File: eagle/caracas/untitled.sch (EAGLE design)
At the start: 12 parts, among them IC1 4027N, Q1 IRFP250

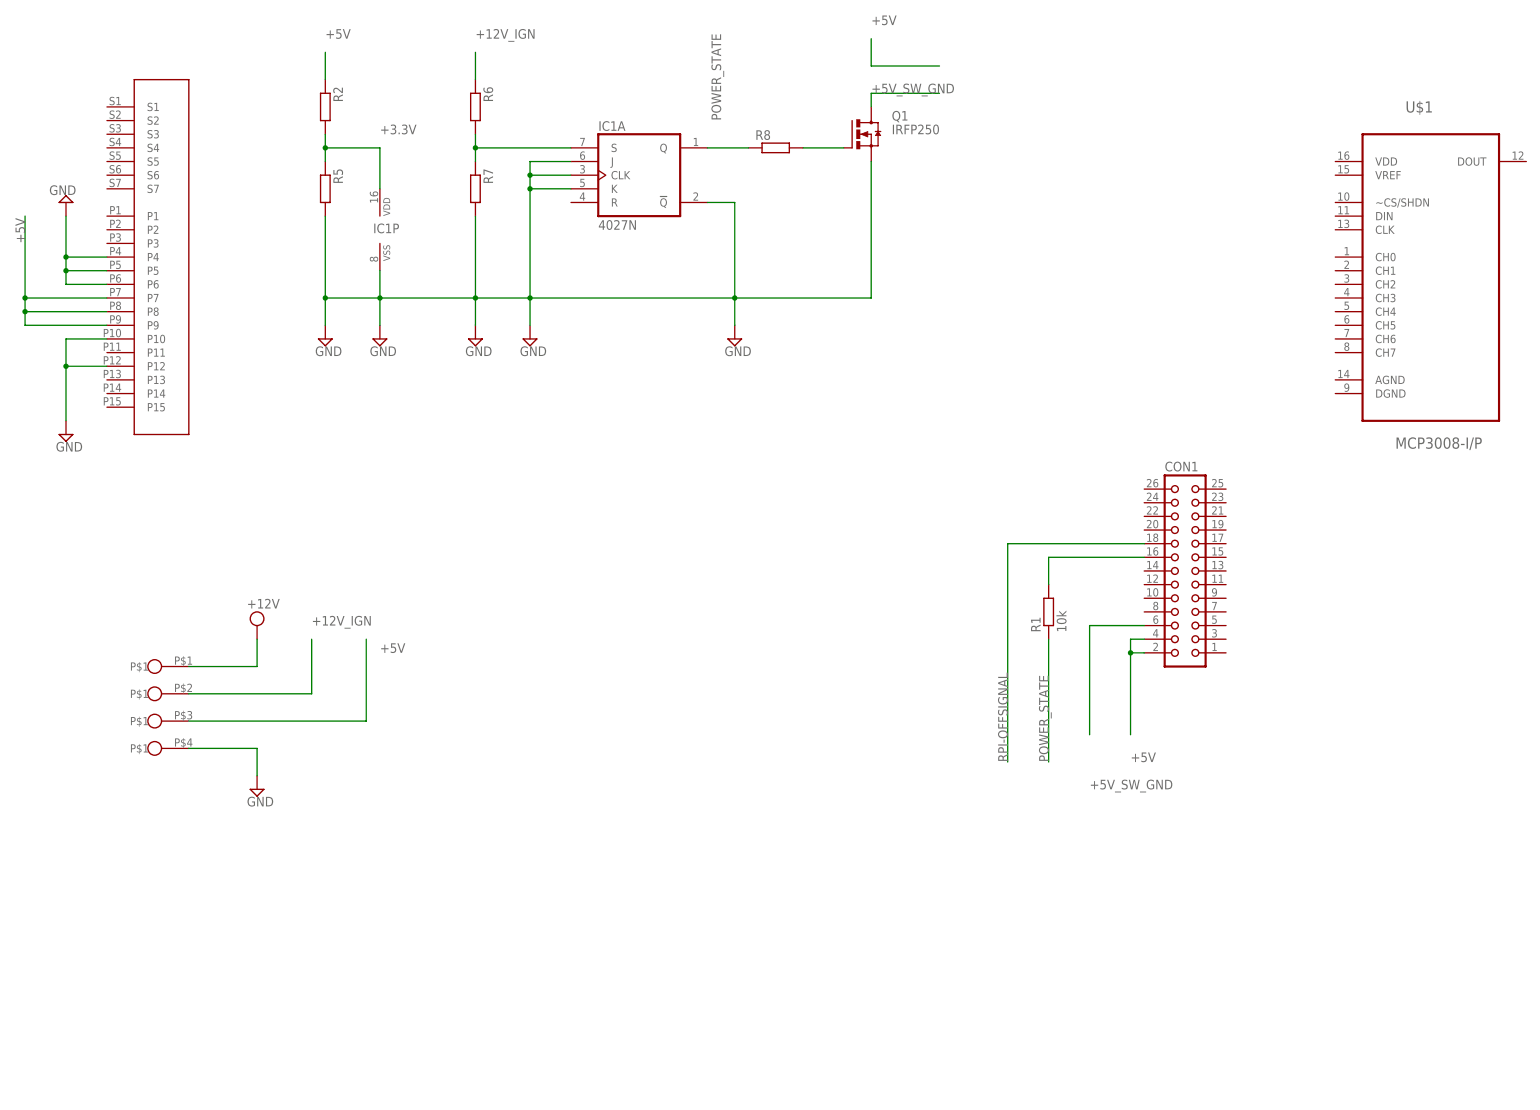
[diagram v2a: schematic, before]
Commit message: WIP on electronics schema.
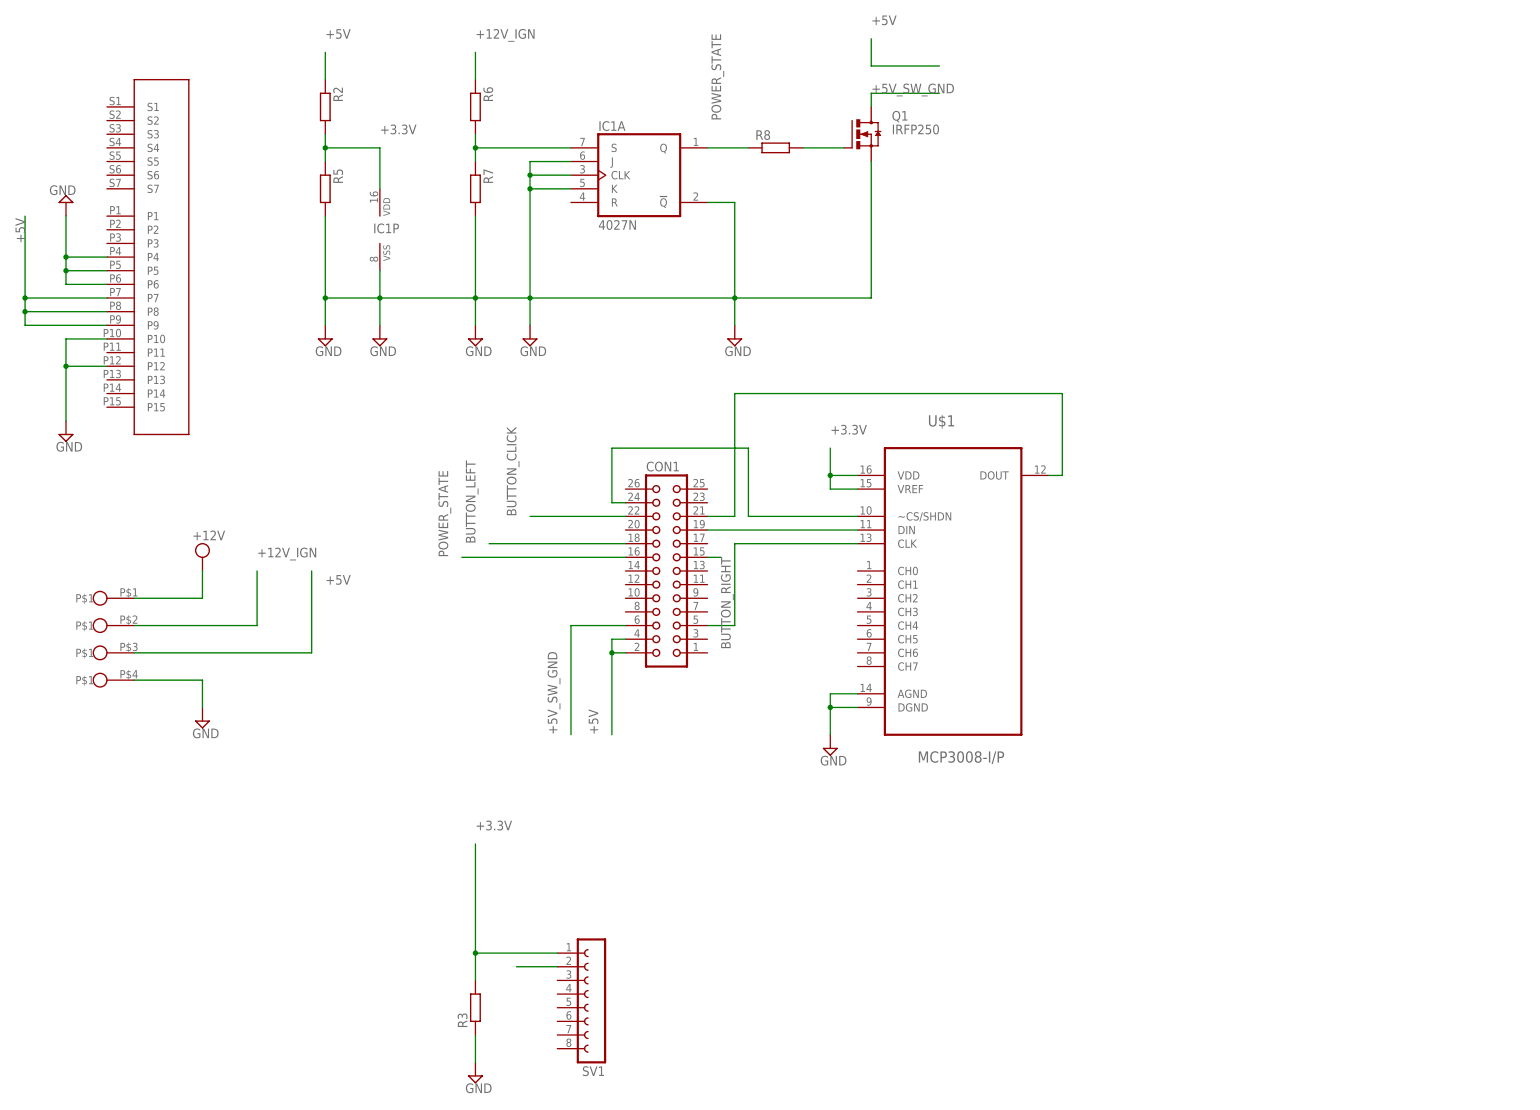
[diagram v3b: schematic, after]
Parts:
- removed R1: 10k, rcl:R-EU_0207/10
- added R3: (no value), rcl:R-EU_0207/10
- added SV1: (no value), con-lsta:FE08-1
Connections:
- net RPI-OFFSIGNAL renamed BUTTON_LEFT
- new net BUTTON_CLICK: CON1.22
- new net BUTTON_RIGHT: CON1.15
- new net N$4: CON1.21, U$1.DOUT
- new net N$5: CON1.19, U$1.DIN
- new net N$6: CON1.24, U$1.~CS/SHDN
- new net N$7: R3.2, SV1.1
- new net N$8: SV1.2
- net +3.3V: now also U$1.VDD, U$1.VREF
- net GND: now also R3.1, U$1.AGND, U$1.DGND
- net N$3: now also CON1.5, U$1.CLK; no longer CON1.16, R1.2
- net POWER_STATE: now also CON1.16; no longer R1.1
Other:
- moved on the sheet: CON1, U$1

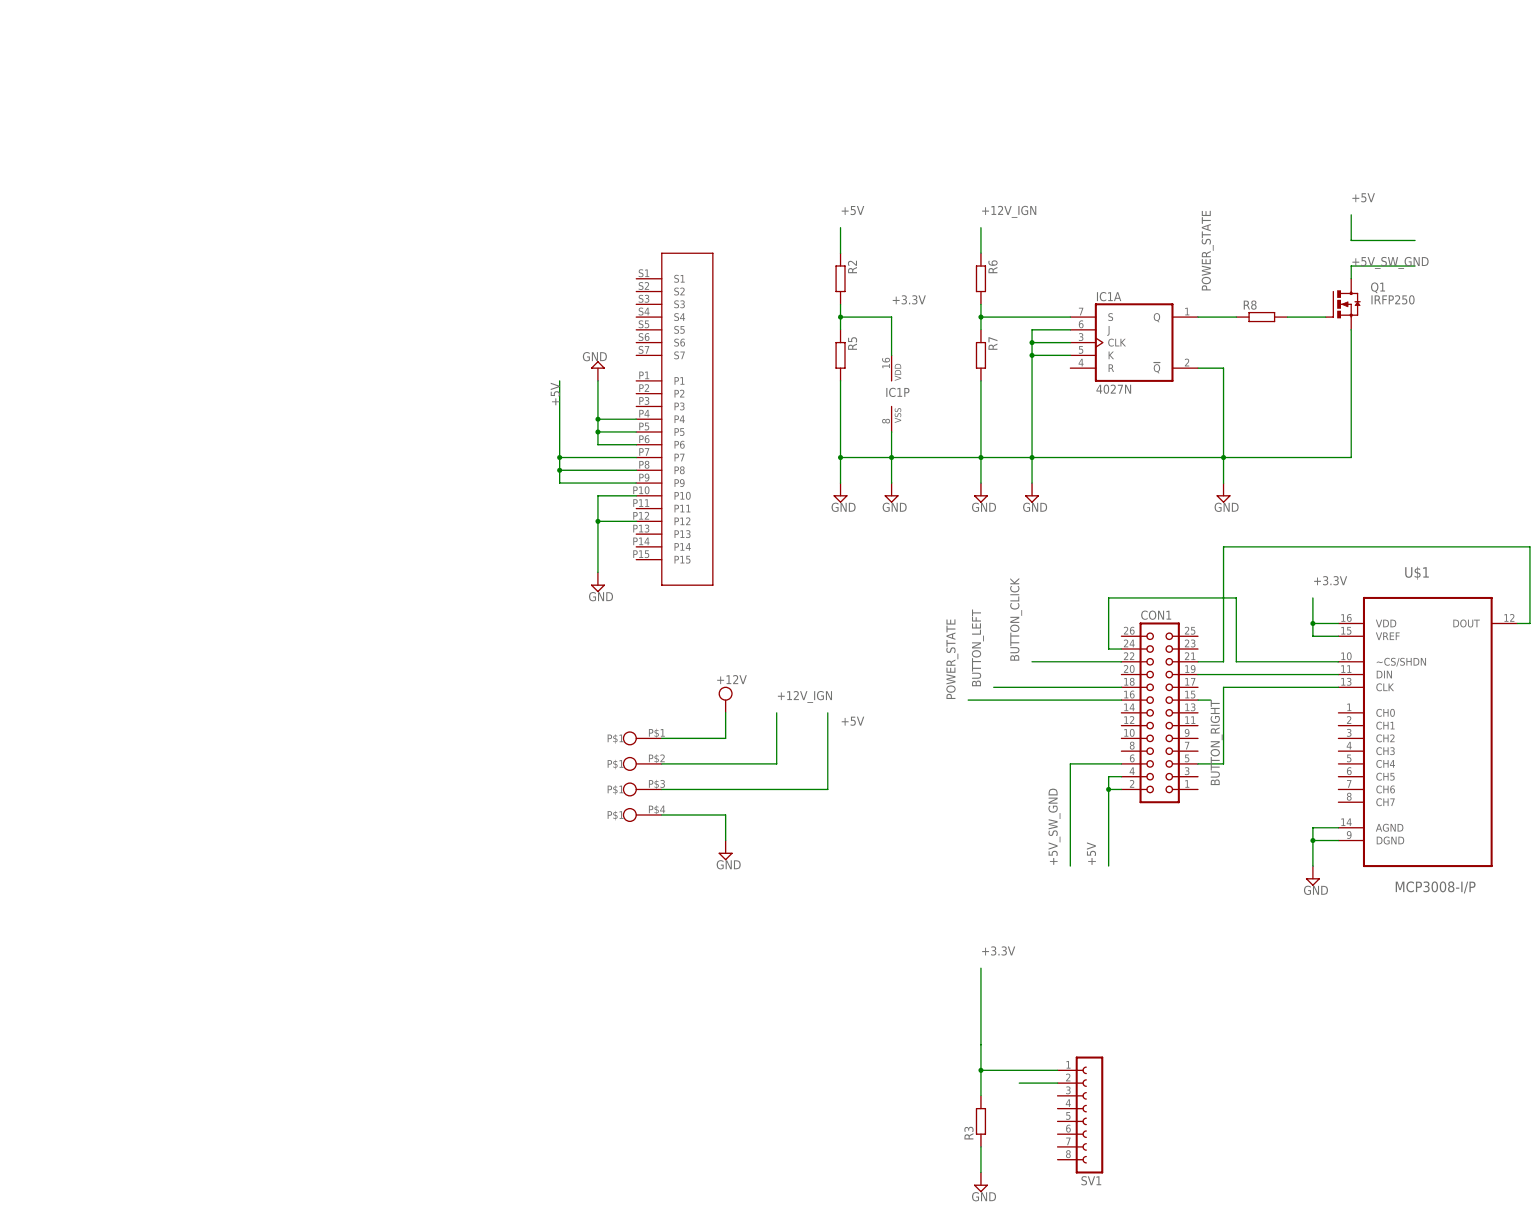
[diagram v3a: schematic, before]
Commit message: More WIP on the electronics schematics, closing in...
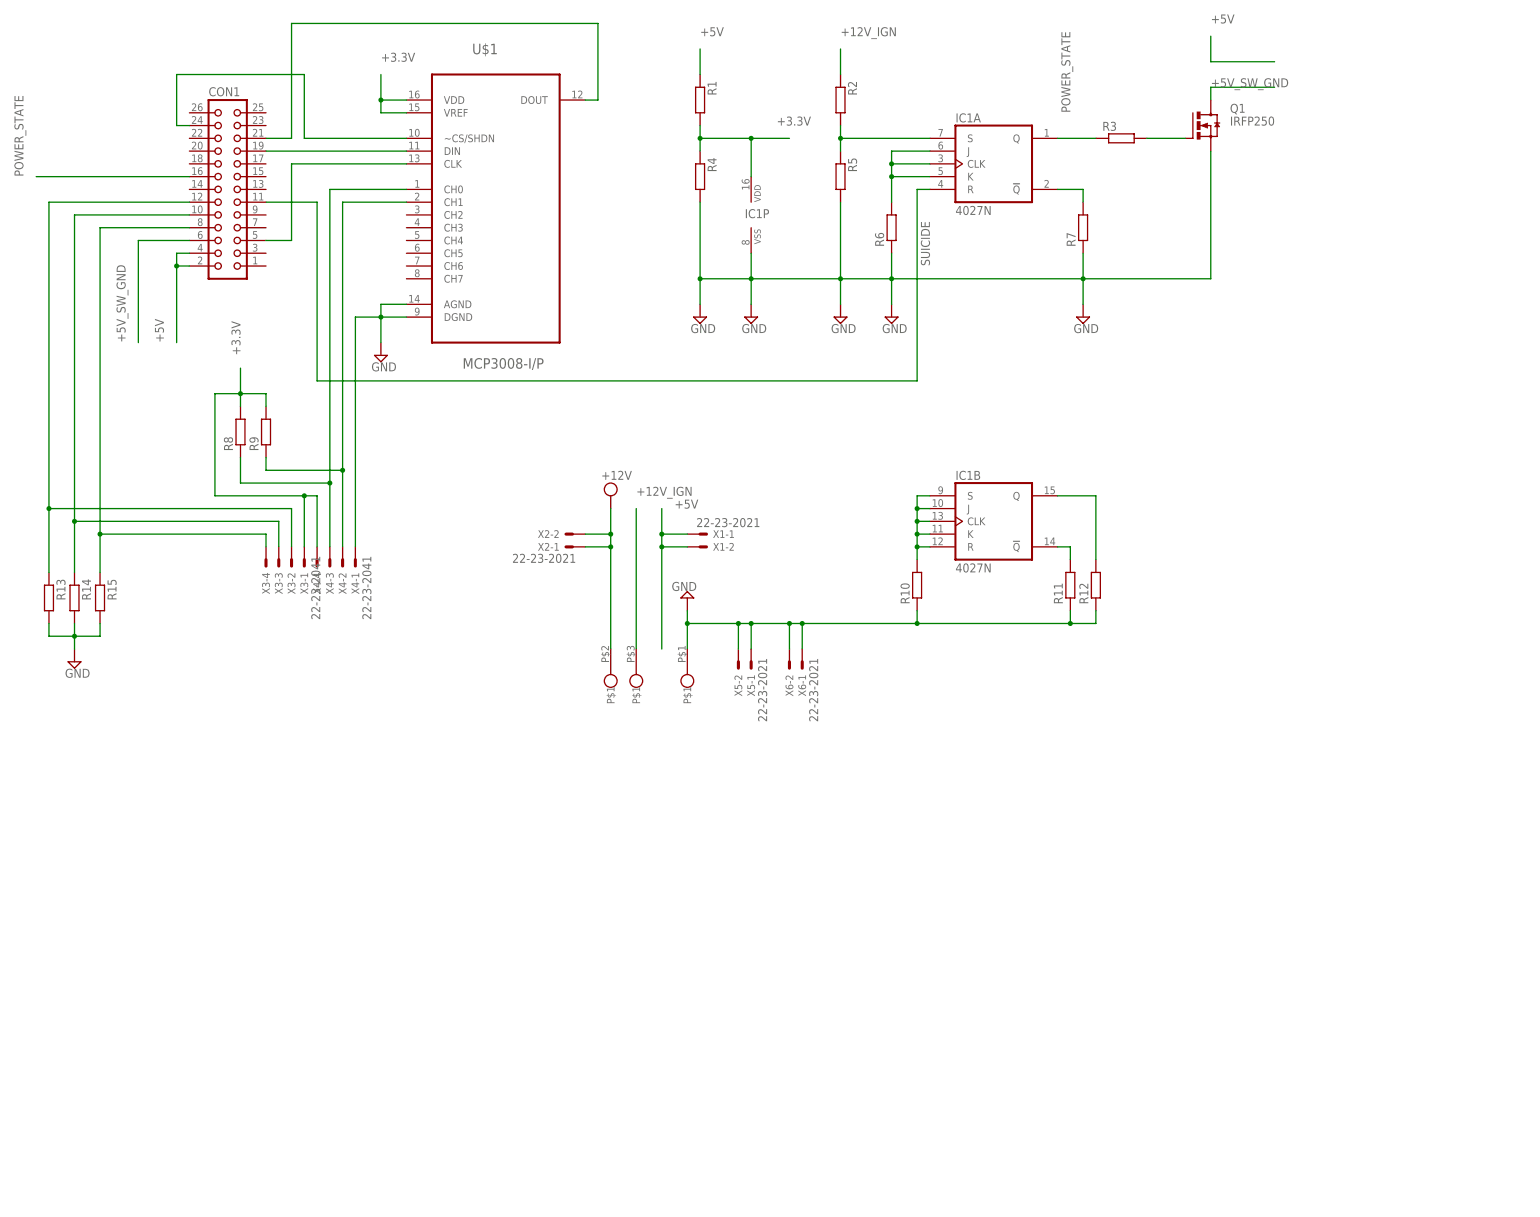
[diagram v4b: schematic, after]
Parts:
- removed SV1: (no value), con-lsta:FE08-1
- removed U$3: MKDS3, caracas:MKDS3
- added R1, R10, R11, R12, R13, R14, R15, R4, R9: (no value), rcl:R-EU_0207/10
- added X1, X2, X5, X6: 22-23-2021, con-molex:22-23-2021
- added X3, X4: 22-23-2041, con-molex:22-23-2041
- U$2: value CD2109 -> MKDS3; device caracas:CD2109 -> caracas:MKDS3
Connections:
- removed net BUTTON_CLICK: CON1.22
- removed net BUTTON_LEFT: CON1.18
- removed net BUTTON_RIGHT: CON1.15
- new net ANA_0: R8.1, U$1.CH0, X4-3.S
- new net ANA_1: R9.1, U$1.CH1, X4-2.S
- new net N$10: CON1.12, R13.1, X3-2.S
- new net N$11: IC1B.!Q, R11.2
- new net N$12: IC1B.CLK, IC1B.J, IC1B.K, IC1B.R, IC1B.S, R10.2
- new net N$13: IC1B.Q, R12.2
- new net N$9: IC1A.CLK, IC1A.J, IC1A.K, R6.2
- new net SUICIDE: CON1.11, IC1A.R
- net +12V_IGN: now also R2.1, U$2G$3.P$1; no longer R6.1, U$3G$2.P$1
- net +3.3V: now also R1.2, R4.1, R8.2, R9.2, X3-1.S, X4-4.S; no longer R2.2, R5.1
- net +3.3V1: now also R2.2, R5.1; no longer R6.2, R7.1
- net +5V: now also R1.1, X1-1.S, X1-2.S; no longer R2.1, U$2.P7, U$2.P8, U$2.P9, U$3G$3.P$1
- net GND: now also R10.1, R11.1, R12.1, R13.2, R14.2, R15.2, R4.2, R6.1, R7.1, U$2G$1.P$1, X4-1.S, X5-1.S, X5-2.S, X6-1.S, X6-2.S; no longer IC1A.CLK, IC1A.J, IC1A.K, R3.1, R7.2, U$2.P10, U$2.P12, U$2.P4, U$2.P5, U$2.P6, U$3G$4.P$1
- net N$1: now also R3.2; no longer R8.2
- net N$2: now also R7.2
- net N$7: now also CON1.8, R15.1, X3-4.S; no longer R3.2, SV1.1
- net N$8: now also CON1.10, R14.1, X3-3.S; no longer SV1.2
- net POWER_STATE: now also R3.1; no longer R8.1
- net VCC: now also U$2G$2.P$1, X2-1.S, X2-2.S; no longer U$3G$1.P$1
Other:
- moved on the sheet: CON1, IC1A, IC1P, Q1, R2, R3, R5, R6, R7, R8, U$1
